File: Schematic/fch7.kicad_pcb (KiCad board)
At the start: 4 copper layers, 39.8 x 41.5 mm, 156 parts, among them IC1 MP9943AGQ-Z, IC2 MP9943AGQ-Z, IC4 ICM-42688-P, IC5 MPU-6500, J1 A-1JB, J1 Conn_Coaxial, J11 PIN2216, J12 PIN2216, J2 PIN2216, J3 PIN2216, J4 PIN2216, J5 PIN2216, J6 PIN2216, J7 PIN2216, J8 PIN2216, J9 PIN2216, U1 ME6217C33M5G, U10 HDGC1002WR-S-4P, U11 HDGC1002WR-S-4P, U12 E28-2G4M27SX, U13 STM32H742VIHx, U14 MIA-M10Q, U15 HDGC1002WR-S-6P, U16 HDGC1002WR-S-8P, U17 HDGC1002WR-S-8P, U18 MAX40200ANS, U2 ME6217C33M5G, U3 LDO-1.8v, U4 QMC5883L, U5 SPL06-001, U6 CSNP1GCR01-BOW, U7 HDGC1002WR-S-6P, U8 HDGC1002WR-S-4P, U9 HDGC1002WR-S-4P, Y1 8MHz, Y2 CM8V-T1A

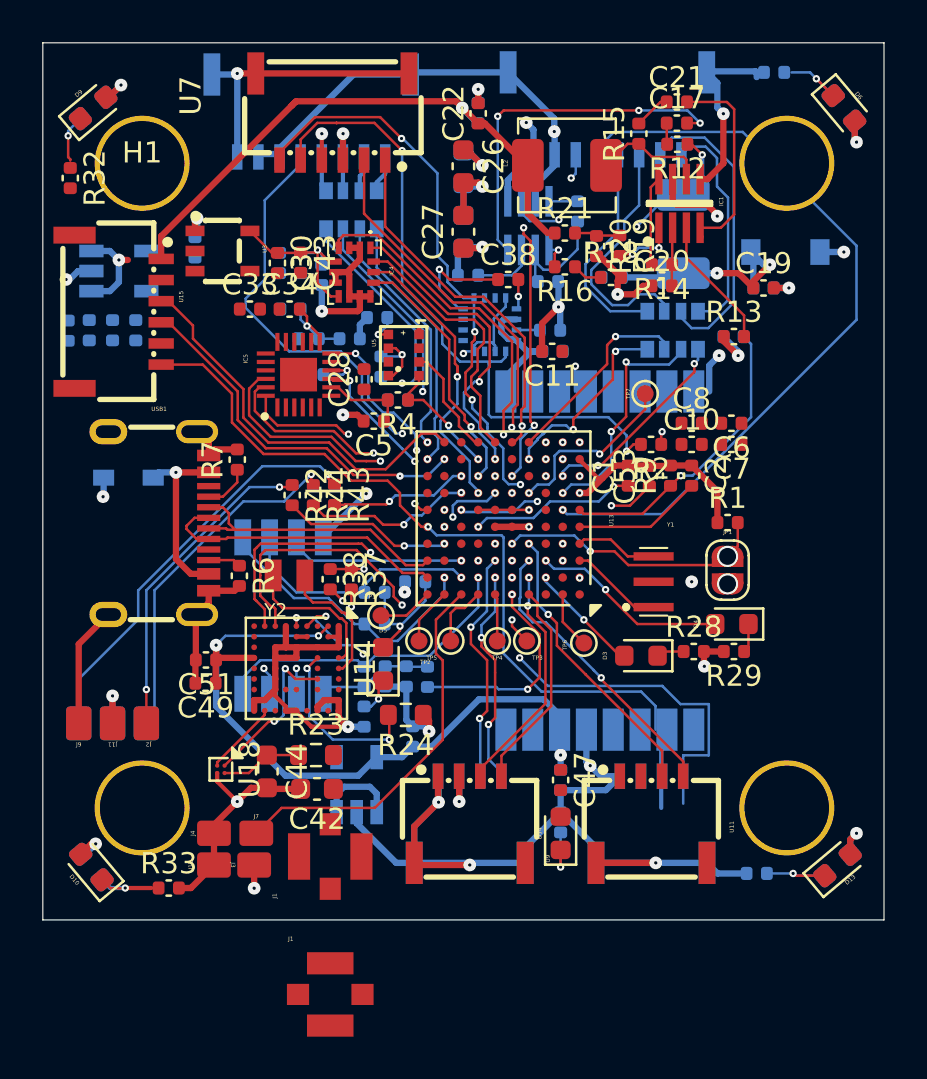
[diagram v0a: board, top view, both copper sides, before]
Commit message: update routing
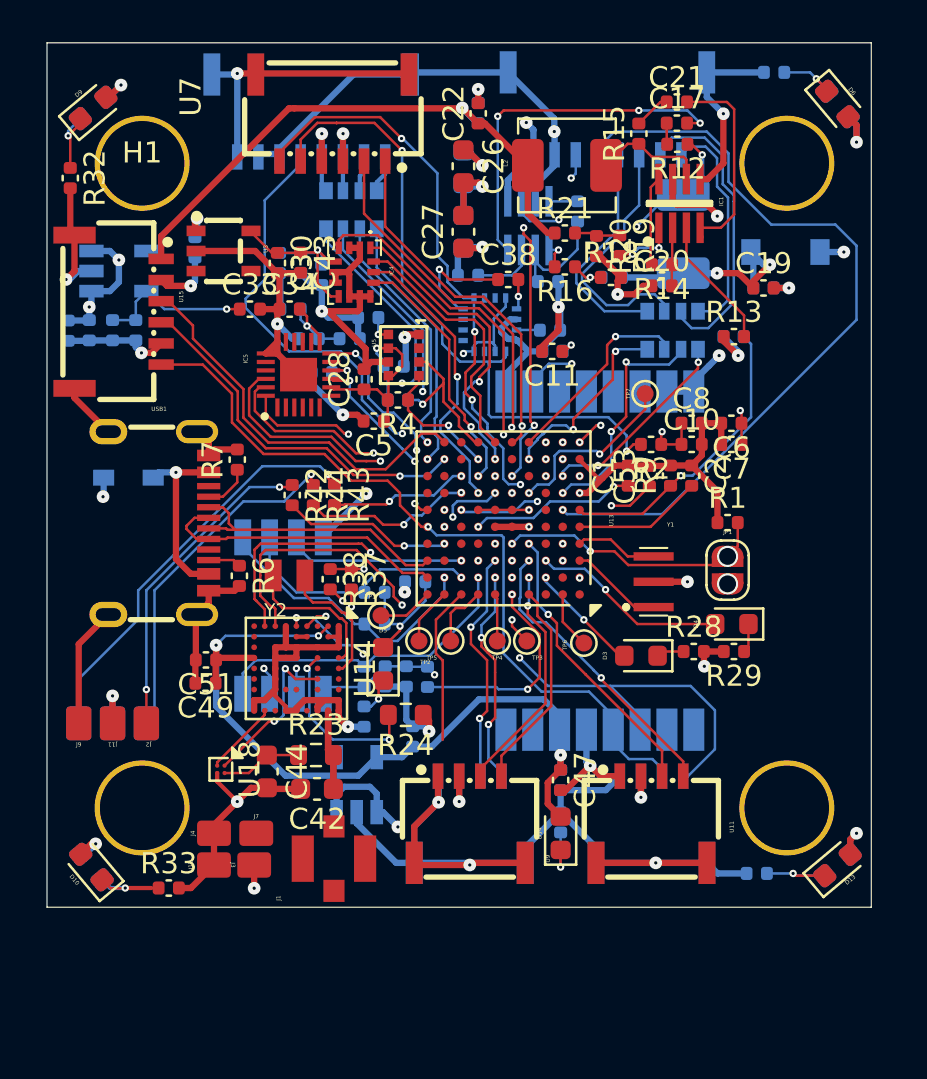
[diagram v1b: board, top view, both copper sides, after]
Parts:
- removed the J1 at (78.0, 105.2)
- removed the J1 at (78.0, 98.7)
- added J1: Conn_Coaxial, fch7:AMPHENOL_A-1JB, F.Cu at (78.2, 98.8)
- moved C29 0.60 mm to (81.0, 75.5), turned to 0 degrees
- moved R22 0.42 mm to (79.8, 73.2)
- moved C32 0.41 mm to (77.6, 75.8)
- moved D6 0.37 mm to (102.0, 63.1)
- moved D7 0.36 mm to (102.0, 63.1)
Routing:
- net GND: track 177.7 -> 238.2 mm, vias 27 -> 31
- net VDD_MCU: track 40.6 -> 57.7 mm, vias 11 -> 16
- net BEEPER: track 18.3 -> 7.61 mm
- net 5V: track 27.3 -> 33.5 mm, vias 12 -> 15
- net /rf_rx/RF_IN: track 0.00 -> 3.80 mm
- net VDD_RECV: track 34.2 -> 37.7 mm
- net I2C2_SDA: track 5.26 -> 7.43 mm, vias 0 -> 1
- net UART6_RX: track 39.0 -> 37.1 mm
- net NRESET_RECV: track 18.3 -> 20.1 mm
- net Net-(D8-K): track 2.27 -> 3.66 mm
- net UART6_TX: track 27.2 -> 28.2 mm
- net VCC_ICM: track 9.36 -> 10.4 mm
- net SENS_CUR1: track 36.4 -> 37.2 mm
- net SPI4_SCLK: track 14.4 -> 13.6 mm
- net Net-(R16-Pad1): track 1.23 -> 1.97 mm, vias 0 -> 1
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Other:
- board size 39.8 x 41.5 mm -> 39 x 40.9 mm

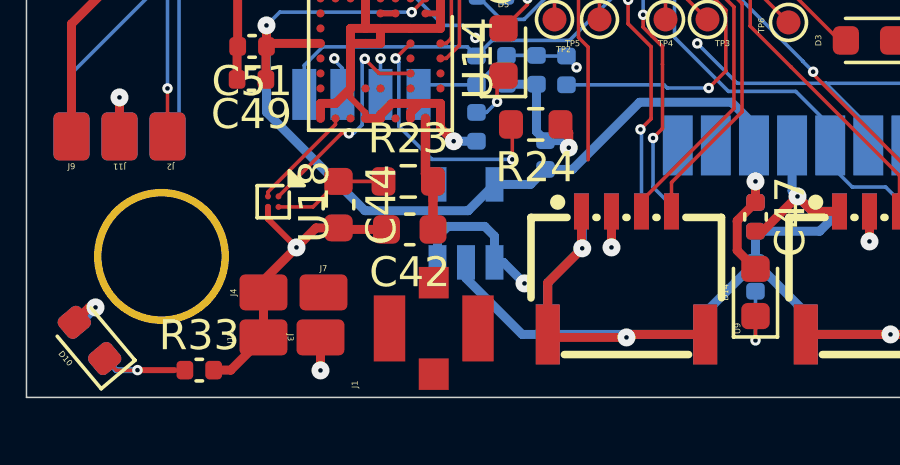
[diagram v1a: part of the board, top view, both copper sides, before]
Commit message: update routing
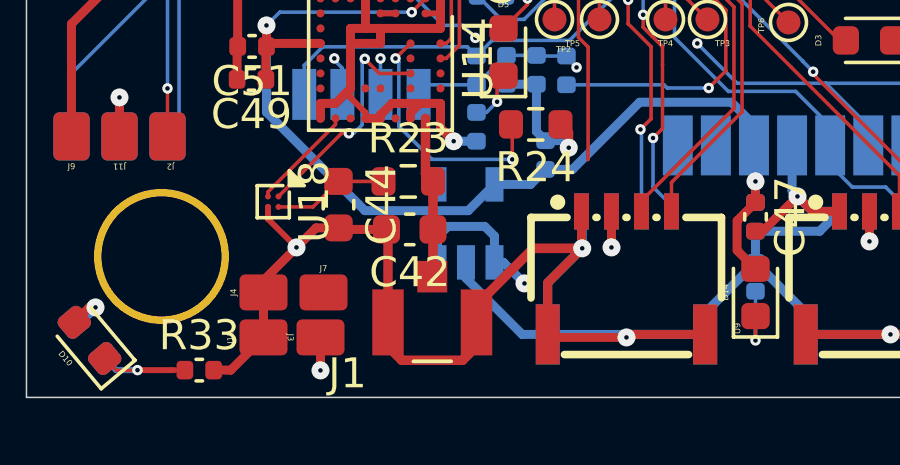
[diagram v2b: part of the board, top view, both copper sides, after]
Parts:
- J1: value Conn_Coaxial -> U.FL-R-SMT-1_01_; footprint fch7:AMPHENOL_A-1JB -> fch7:HIROSE_U.FL-R-SMT-1_01_
- moved J1 0.21 mm to (78.1, 98.6), turned to 180 degrees
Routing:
- net GND: track 238.2 -> 251.1 mm
- net /rf_rx/RF_IN: track 3.80 -> 5.39 mm
